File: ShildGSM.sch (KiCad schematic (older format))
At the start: 33 parts, among them P1 Power, P10 CONN_01X05, P14 CONN_01X07, P15 CONN_1, P16 CONN_1, P2 Analog, P3 Digital, P4 Digital, P5 CONN_1, P6 CONN_1, P8 CONN_1, P9 CONN_01X05, U1 LM2567T-5

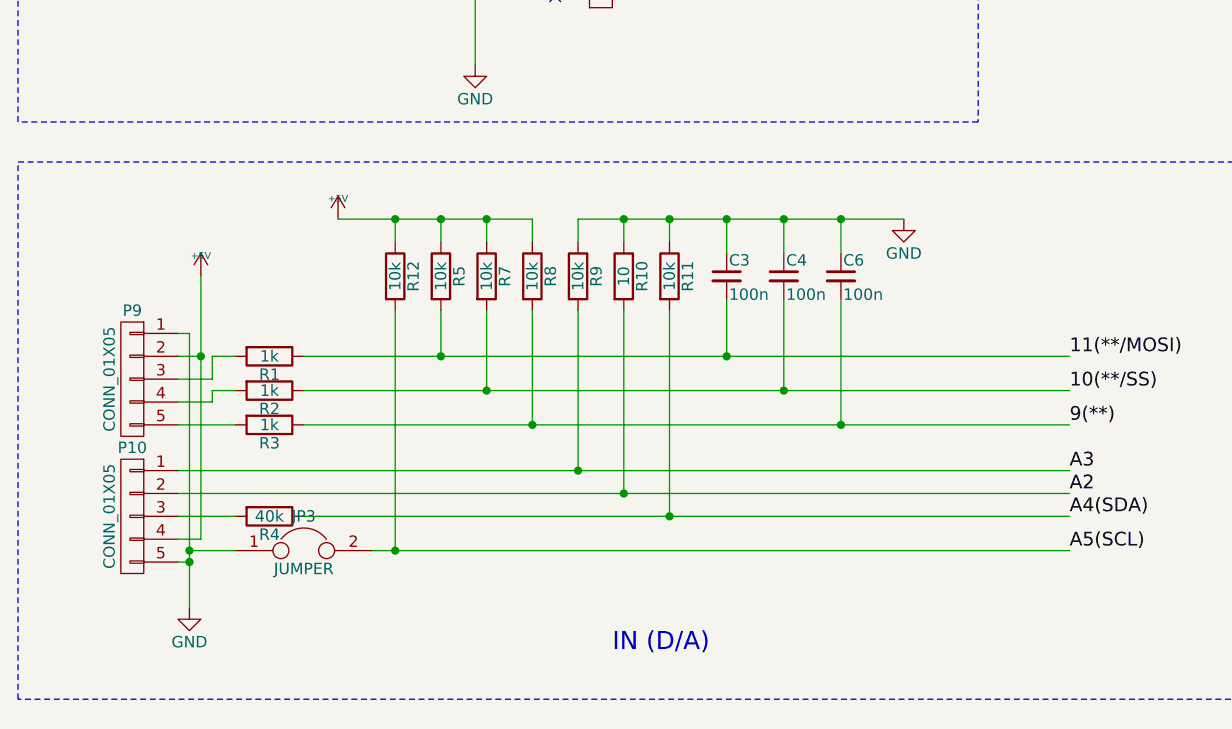
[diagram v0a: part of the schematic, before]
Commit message: corectii
corectii in schema
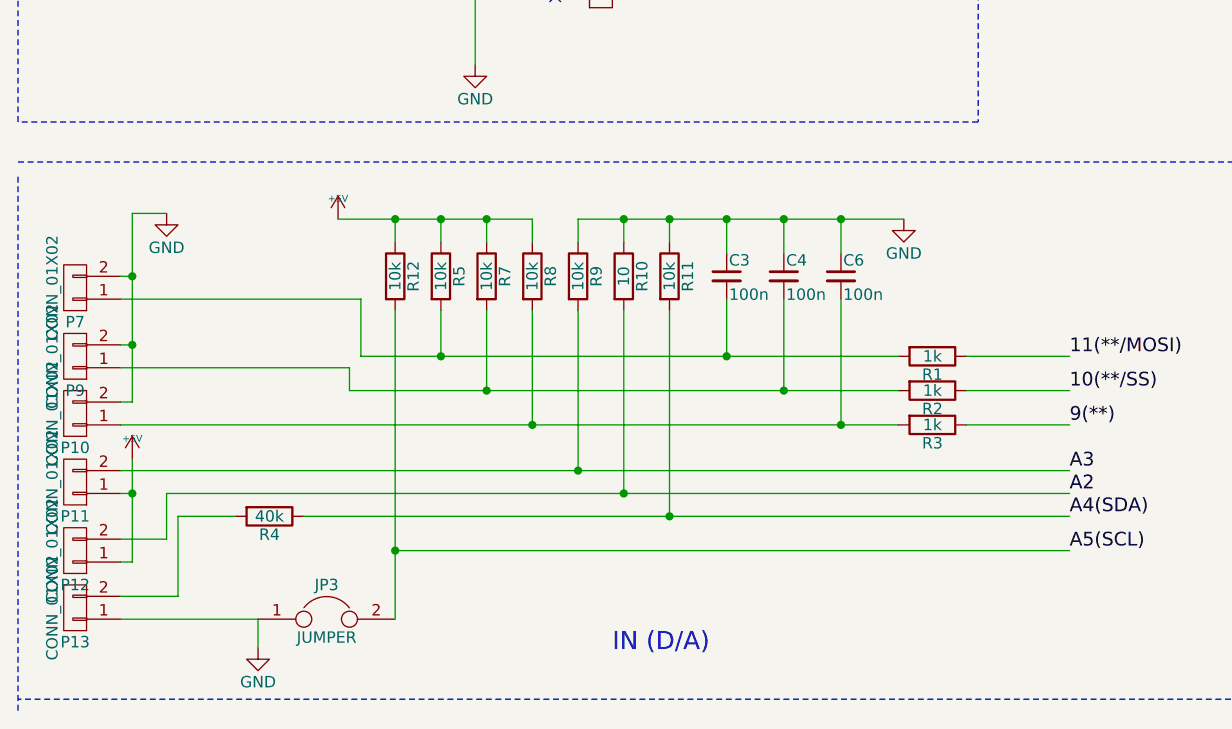
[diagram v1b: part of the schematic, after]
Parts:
- removed P10: CONN_01X05, Terminal_Blocks:TerminalBlock_Pheonix_PT-3.5mm_5pol, symbol CONN_01X05
- removed P9: CONN_01X05, Terminal_Blocks:TerminalBlock_Pheonix_PT-3.5mm_4pol, symbol CONN_01X05
- added P10, P11, P12, P13, P7, P9: CONN_01X02, Sockets_MOLEX_KK-System:Socket_MOLEX-KK-RM2-54mm_Lock_2pin_straight, symbol CONN_01X02
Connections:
- wire segments 105 -> 112
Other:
- moved on the sheet: JP3, R1, R2, R3

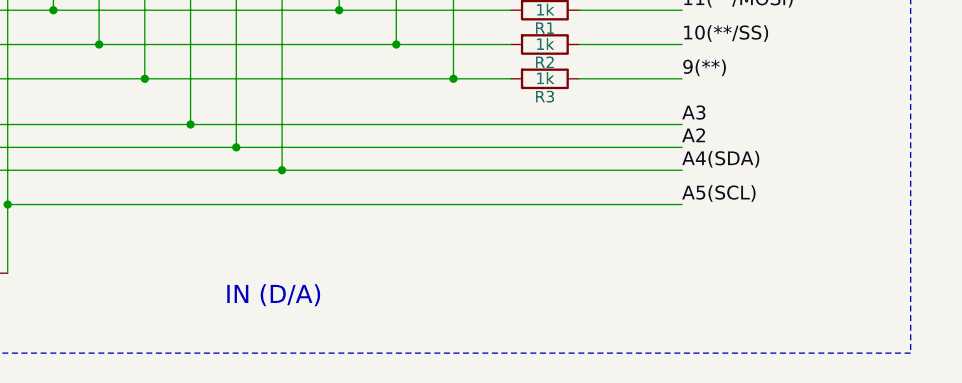
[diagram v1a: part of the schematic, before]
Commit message: LEDs
pus led err si led use
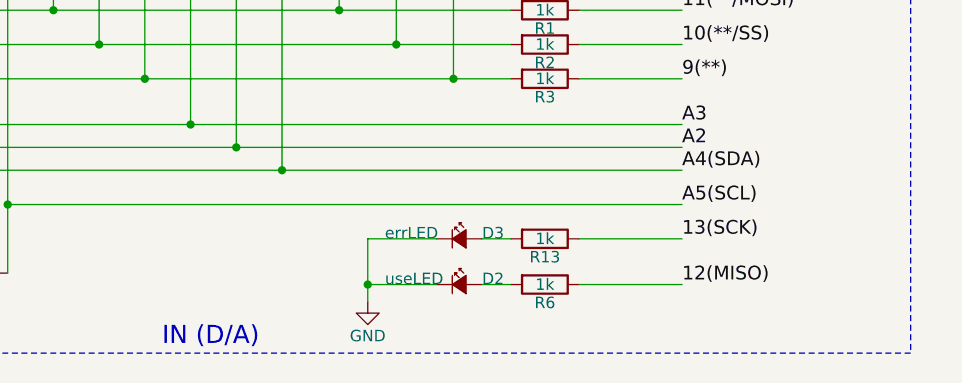
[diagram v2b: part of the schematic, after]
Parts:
- added D2: useLED, LEDs:LED-3MM, symbol Led_Small
- added D3: errLED, LEDs:LED-3MM, symbol Led_Small
- added R13, R6: 1k, Discret:R3, symbol R
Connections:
- wire segments 112 -> 119
